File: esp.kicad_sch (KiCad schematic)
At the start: 30 parts, among them J1 Barrel_Jack, J2 8P8C_Shielded, J21 8P8C_Shielded, J3 Barrel_Jack, J38 8P8C_Shielded, J4 Barrel_Jack, J5 Barrel_Jack, J7 Barrel_Jack_MountingPin, K1 RT314A24, P1 Conn_WallPlug_Earth, U1 ESP32-S2-WROVER, U14 PCF8574ATS, U16 L298N, U17 PCA9685PW, U18 NID30S48-24, U2 TCA9548ARGER, U3 TCA9548ARGER, U4 BME280, U5 CCS811, U6 PCF8574ATS, U7 OKI-78SR-12_1.0-W36H-C, U8 OKI-78SR-5_1.5-W36-C, U9 OKI-78SR-3.3_1.5-W36H-C

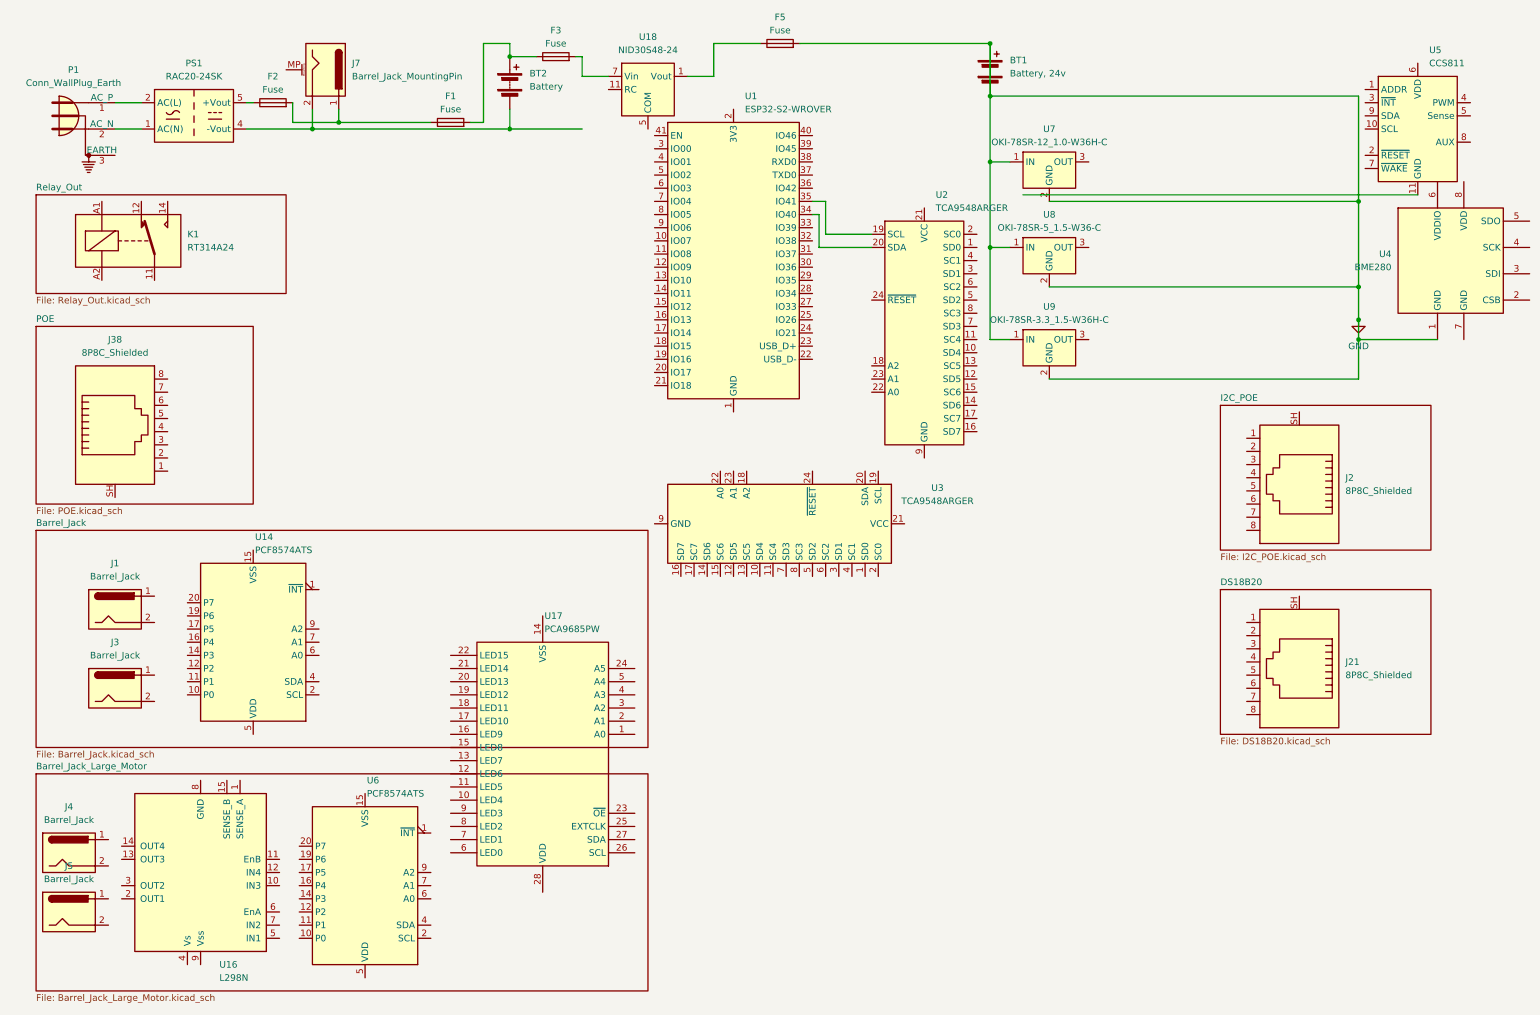
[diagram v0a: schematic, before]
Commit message: some relay adjustments
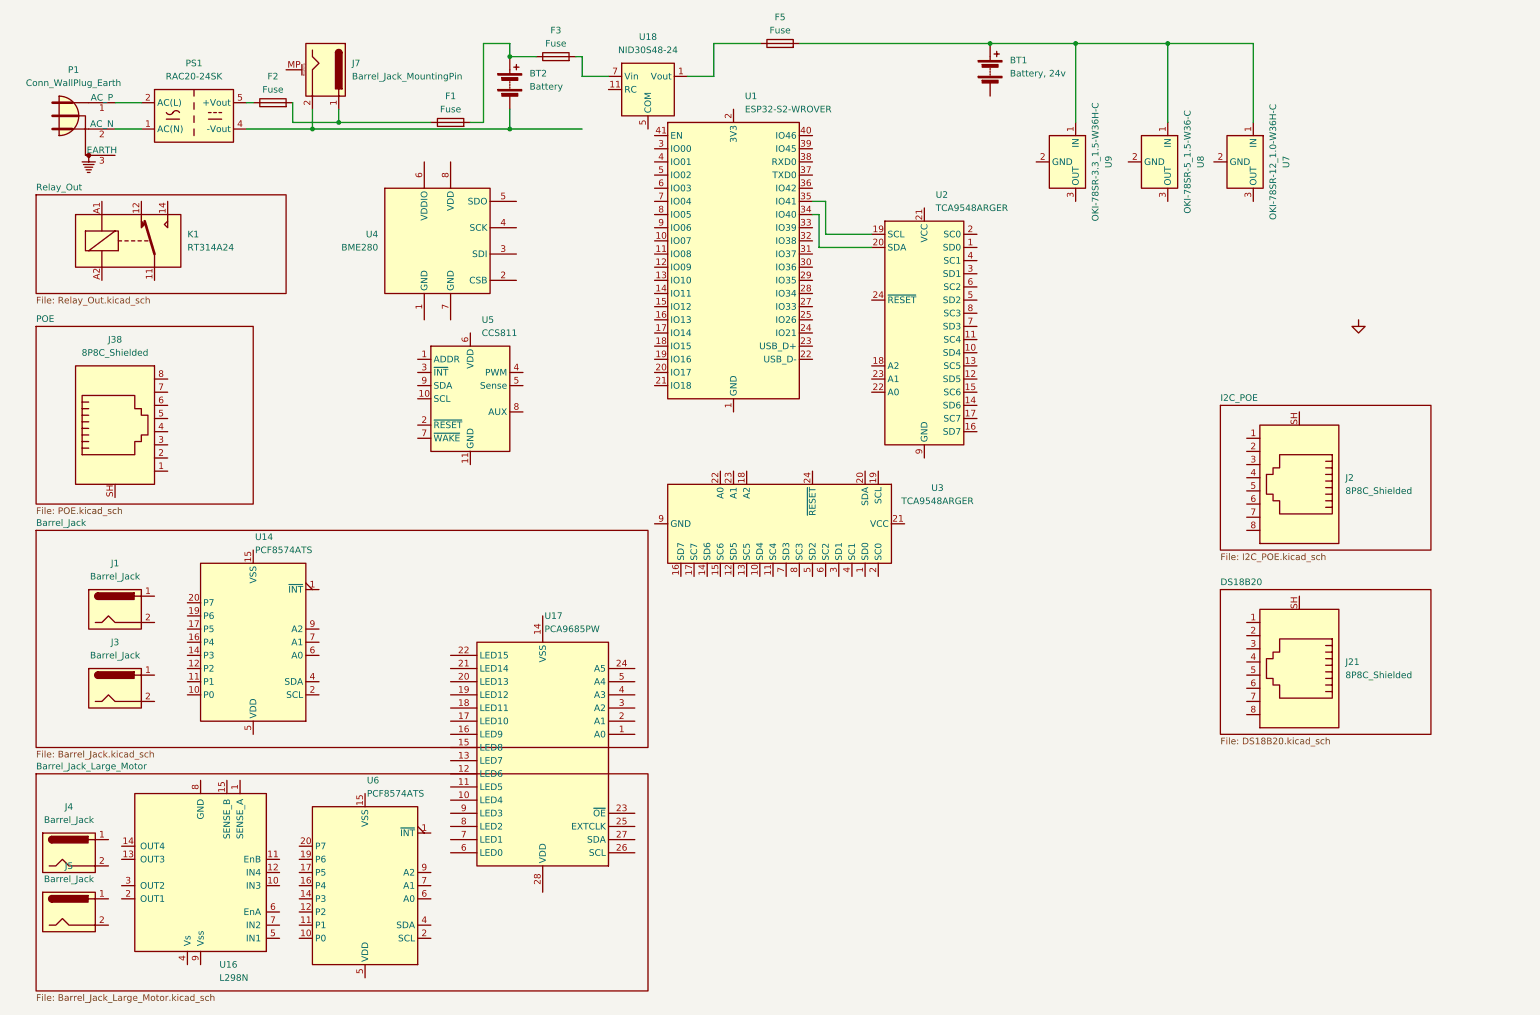
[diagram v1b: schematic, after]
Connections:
- net GND: no longer BT1.1 (+), BT1.2 (-), F5.2, U4.1 (GND), U7.1 (IN), U7.2 (GND), U8.1 (IN), U8.2 (GND), U9.1 (IN), U9.2 (GND)
- new net: BT1.1 (+), F5.2, U7.1 (IN), U8.1 (IN), U9.1 (IN)
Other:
- moved on the sheet: U4, U5, U7, U8, U9
